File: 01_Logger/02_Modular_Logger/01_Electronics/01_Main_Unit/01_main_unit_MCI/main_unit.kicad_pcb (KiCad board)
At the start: 4 copper layers, 54.9 x 27.4 mm, 34 parts, among them J1 Conn_01x02, J102 FTS-107-01-F-D, J2 Conn_01x04_Pin, J3 Conn_01x04_Pin, J301 Conn_01x02, J302 Conn_02x04_Counter_Clockwise, J304 Conn_02x02_Odd_Even, J701 Micro_SD_Card_Det, SW301 SW_Push, U301 MAX16125WTEG00+T, U302 ESP32-S3-WROOM-1U, U303 DS3231MZ, Y301 Crystal

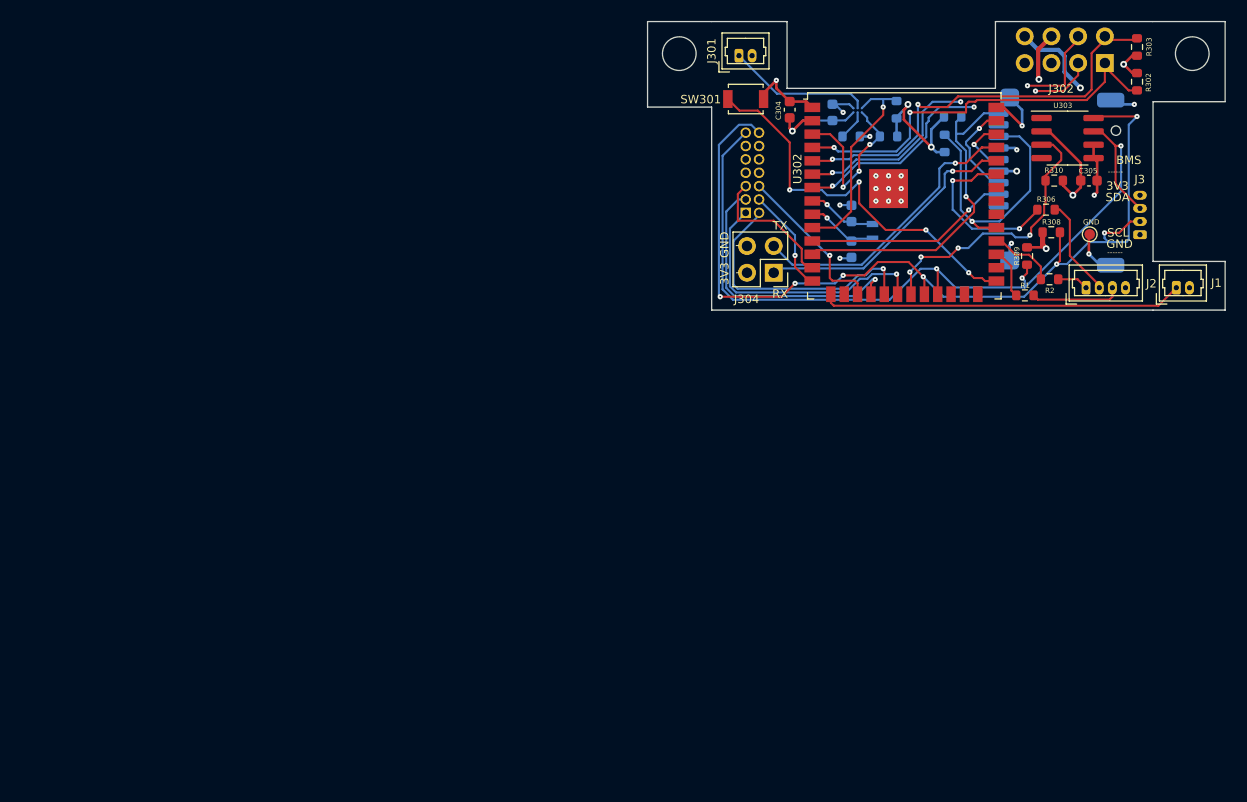
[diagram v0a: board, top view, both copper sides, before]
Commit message: Main_Unit Update
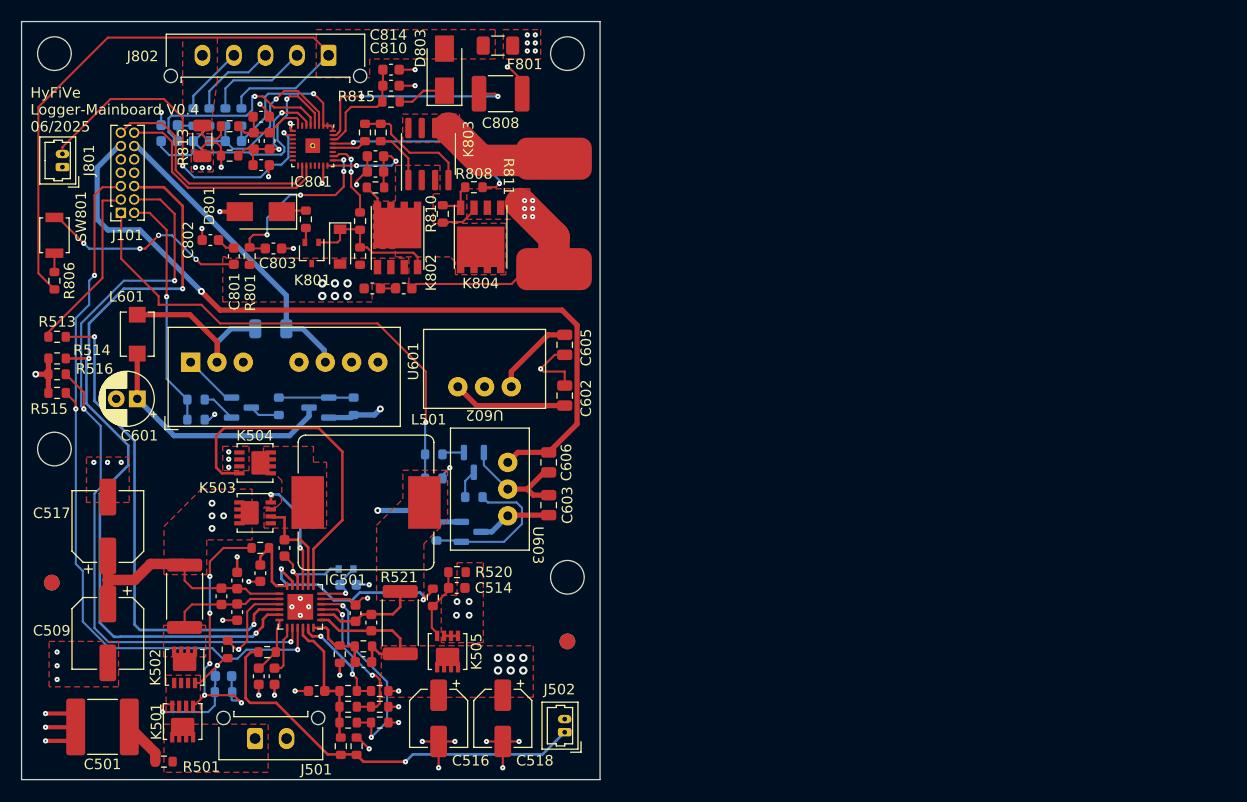
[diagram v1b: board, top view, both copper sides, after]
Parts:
- removed C301, C302: 20pF, Capacitor_SMD:C_0603_1608Metric
- removed C303, C304, C305: 100nF 50V, Capacitor_SMD:C_0603_1608Metric
- removed H303, H305: MountingHole, MountingHole:MountingHole_3.2mm_M3_ISO7380
- removed J1, J301: Conn_01x02, Connector_Molex:Molex_PicoBlade_53047-0210_1x02_P1.25mm_Vertical
- removed J102: FTS-107-01-F-D, Connector_PinHeader_1.27mm:PinHeader_2x07_P1.27mm_Vertical
- removed J2, J3: Conn_01x04_Pin, Connector_Molex:Molex_PicoBlade_53047-0410_1x04_P1.25mm_Vertical
- removed J302: Conn_02x04_Counter_Clockwise, Connector_PinHeader_2.54mm:PinHeader_2x04_P2.54mm_Horizontal
- removed J304: Conn_02x02_Odd_Even, Connector_PinHeader_2.54mm:PinHeader_2x02_P2.54mm_Vertical
- removed J701: Micro_SD_Card_Det, HER_Footprints:SD_CARD_693071020811
- removed R1, R2: 0R, Resistor_SMD:R_0603_1608Metric
- removed R301: 470k, Resistor_SMD:R_0603_1608Metric
- removed R302, R303, R304, R305, R308, R309, R310, R701, R702: 10k, Resistor_SMD:R_0603_1608Metric
- removed R306: 68R, Resistor_SMD:R_0603_1608Metric
- removed SW301: SW_Push, Button_Switch_SMD:SW_SPST_B3U-1000P
- removed TP303: TestPoint, TestPoint:TestPoint_Pad_D1.0mm
- removed U301: MAX16125WTEG00+T, MAX6071ANT25_T:WLP-6
- removed U302: ESP32-S3-WROOM-1U, HER_Footprints:ESP32-S3-WROOM-1U
- removed U303: DS3231MZ, Package_SO:SOIC-8_3.9x4.9mm_P1.27mm
- removed Y301: Crystal, Crystal:Crystal_SMD_TXC_9HT11-2Pin_2.0x1.2mm
- added C501: 47µF 35V X7R, Capacitor_SMD:C_2220_5650Metric, F.Cu at (107.7, 145.3)
- added C502: 100nF 50V, Capacitor_SMD:C_0603_1608Metric, B.Cu at (119.2, 140.5)
- added C503: 100nF 50V, Capacitor_SMD:C_0603_1608Metric, F.Cu at (120.5, 134.4)
- added C504: 1µF 10V, Capacitor_SMD:C_0603_1608Metric, F.Cu at (128.1, 141.9)
- added C505: 100nF 50V, Capacitor_SMD:C_0603_1608Metric, F.Cu at (119.0, 132.9)
- added C506: 100nF 50V, Capacitor_SMD:C_0603_1608Metric, F.Cu at (122.5, 140.5)
- added C507: 100nF 50V, Capacitor_SMD:C_0603_1608Metric, F.Cu at (120.5, 131.4)
- added C508: 33nF 25V, Capacitor_SMD:C_0603_1608Metric, F.Cu at (124.0, 140.5)
- added C509: 47µF 35V, Capacitor_SMD:CP_Elec_6.3x5.4, F.Cu at (108.2, 136.4)
- added C510: 1µF 35V, Capacitor_SMD:C_0603_1608Metric, F.Cu at (122.7, 130.7)
- added C511: 100nF 50V, Capacitor_SMD:C_0603_1608Metric, F.Cu at (125.0, 128.3)
- added C512: 1µF 35V, Capacitor_SMD:C_0603_1608Metric, B.Cu at (131.1, 131.8)
- added C513: 100nF 50V, Capacitor_SMD:C_0603_1608Metric, F.Cu at (131.8, 134.5)
- added C514: 100nF 50V, Capacitor_SMD:C_0603_1608Metric, F.Cu at (141.4, 132.1)
- added C515: 100nF 50V, Capacitor_SMD:C_0603_1608Metric, F.Cu at (133.2, 135.4)
- added C516: 20µF 35V, Capacitor_SMD:CP_Elec_5x5.3, F.Cu at (139.7, 144.5)
- added C517: 47µF 35V, Capacitor_SMD:CP_Elec_6.3x5.4, F.Cu at (108.2, 126.2)
- added C518: 20µF 35V, Capacitor_SMD:CP_Elec_5x5.3, F.Cu at (145.8, 144.5)
- added C519: 22pF 35V, Capacitor_SMD:C_0603_1608Metric, F.Cu at (132.5, 139.1)
- added C601: 10µF, 50V, Capacitor_THT:CP_Radial_D5.0mm_P2.00mm, F.Cu at (111.0, 114.1)
- added C602: 22µF 30V, Capacitor_SMD:C_0805_2012Metric, F.Cu at (151.6, 113.8)
- added C603: 22µF 30V, Capacitor_SMD:C_0805_2012Metric, F.Cu at (150.1, 124.2)
- added C604: 150pF, 2kV, Capacitor_SMD:C_1206_3216Metric, B.Cu at (123.7, 107.4)
- added C605: 47µF 10V, Capacitor_SMD:C_0805_2012Metric, F.Cu at (151.6, 109.0)
- added C606: 47µF 10V, Capacitor_SMD:C_0805_2012Metric, F.Cu at (150.1, 120.1)
- added C801: 100nF 50V, Capacitor_SMD:C_0603_1608Metric, F.Cu at (120.2, 100.5)
- added C802: 100nF 50V, Capacitor_SMD:C_0603_1608Metric, F.Cu at (117.9, 99.0)
- added C803: 10nF, 50V, Capacitor_SMD:C_0603_1608Metric, F.Cu at (123.9, 99.8)
- added C804: 100pF 50V, Capacitor_SMD:C_0603_1608Metric, F.Cu at (133.6, 92.5)
- added C805: 100pF 50V, Capacitor_SMD:C_0603_1608Metric, F.Cu at (133.6, 91.0)
- added C806: 100nF 50V, Capacitor_SMD:C_0603_1608Metric, F.Cu at (133.3, 103.6)
- added C807: 100nF 50V, Capacitor_SMD:C_0603_1608Metric, F.Cu at (136.3, 103.6)
- added C808: 2,2µF 100V, Capacitor_SMD:C_1812_4532Metric, F.Cu at (145.5, 85.1)
- added C809: 100nF 50V, Capacitor_SMD:C_0603_1608Metric, F.Cu at (122.8, 91.9)
- added C810: 100pF 50V, Capacitor_SMD:C_0603_1608Metric, F.Cu at (135.1, 84.3)
- added C811: 100pF 100V, Capacitor_SMD:C_0603_1608Metric, F.Cu at (123.6, 89.6)
- added C812: 100nF 50V, Capacitor_SMD:C_0603_1608Metric, F.Cu at (122.1, 89.6)
- added C813: 100nF 50V, Capacitor_SMD:C_0603_1608Metric, F.Cu at (122.8, 87.3)
- added C814: 100pF 50V, Capacitor_SMD:C_0603_1608Metric, F.Cu at (135.1, 82.8)
- added C815: 100nF 50V, Capacitor_SMD:C_0603_1608Metric, B.Cu at (120.1, 89.6)
- added C816: 100nF 50V, Capacitor_SMD:C_0603_1608Metric, B.Cu at (117.1, 89.6)
- added C817: 100nF 50V, Capacitor_SMD:C_0603_1608Metric, B.Cu at (114.0, 89.6)
- added C818: 100nF 50V, Capacitor_SMD:C_0603_1608Metric, B.Cu at (114.0, 88.1)
- added D501: BAT54W, Diode_SMD:D_SOD-523, B.Cu at (130.8, 130.3)
- added D801: SS1H10-E3/61T, Diode_SMD:D_SMA, F.Cu at (122.7, 96.3)
- added D802: MMSZ5246B-7-F, Diode_SMD:D_SOD-123, F.Cu at (130.3, 99.6)
- added D803: SS1H10-E3/61T, Diode_SMD:D_SMA, F.Cu at (140.2, 82.8)
- added F801: 12A, Fuse:Fuse_1206_3216Metric, F.Cu at (145.3, 80.5)
- added FID301: Fiducial, Sonstiges:Passmarke, F.Cu at (151.9, 137.2)
- added FID302: Fiducial, Sonstiges:Passmarke, F.Cu at (102.9, 131.6)
- added FID303: Fiducial, Sonstiges:Passmarke, B.Cu at (102.9, 131.6)
- added FID304: Fiducial, Sonstiges:Passmarke, B.Cu at (151.9, 137.2)
- added H301: MountingHole, MountingHole:MountingHole_3.2mm_M3_ISO7380, F.Cu at (103.1, 81.3)
- added H302: MountingHole, MountingHole:MountingHole_3.2mm_M3_ISO7380, F.Cu at (151.9, 81.3)
- added H304: MountingHole, MountingHole:MountingHole_3.2mm_M3_ISO7380, F.Cu at (151.9, 131.1)
- added H306: MountingHole, MountingHole:MountingHole_3.2mm_M3_ISO7380, F.Cu at (103.1, 118.9)
- added IC501: BQ24618, Package_DFN_QFN:VQFN-24-1EP_4x4mm_P0.5mm_EP2.45x2.45mm, F.Cu at (126.5, 133.9)
- added IC801: BQ40Z80, Texas:RSM32 VQFN-32-1EP_4x4mm_P0.4mm_EP1.4x1.4mm_ThermalVias, F.Cu at (127.7, 90.0)
- added J101: SFMC-107-01-L-D, Connector_PinSocket_1.27mm:PinSocket_2x07_P1.27mm_Vertical, F.Cu at (109.4, 96.4)
- added J501: Conn_01x02, Connector_Molex:Molex_Micro-Fit_3.0_43650-0215_1x02_P3.00mm_Vertical, F.Cu at (122.2, 146.4)
- added J502: Conn_01x02_Female, Connector_Molex:Molex_PicoBlade_53047-0210_1x02_P1.25mm_Vertical, F.Cu at (151.6, 145.8)
- added J801: Conn_01x02_Male, Connector_Molex:Molex_PicoBlade_53047-0210_1x02_P1.25mm_Vertical, F.Cu at (103.9, 92.1)
- added J802: Conn_01x05_Male, Connector_Molex:Molex_Micro-Fit_3.0_43650-0515_1x05_P3.00mm_Vertical, F.Cu at (129.2, 81.4)
- added K501: SISH101DN-T1-GE3, Vishay:PowerPAK 1212-8 Single, F.Cu at (115.3, 144.8)
- added K502: SISH101DN-T1-GE3, Vishay:PowerPAK 1212-8 Single, F.Cu at (115.5, 139.6)
- added K503: SiS412DN, Vishay:PowerPAK 1212-8 Single, F.Cu at (122.2, 124.9)
- added K504: SiS412DN, Vishay:PowerPAK 1212-8 Single, F.Cu at (122.2, 120.2)
- added K505: SISH101DN-T1-GE3, Vishay:PowerPAK 1212-8 Single, F.Cu at (140.5, 138.1)
- added K801: 2N7002KW, Package_TO_SOT_SMD:SOT-323_SC-70, F.Cu at (127.6, 100.2)
- added K802: CSD18540Q5B, HER_Footprints:TI Q5B-Package, F.Cu at (135.7, 98.8)
- added K803: DMP6023LSS-13, Package_SO:SOIC-8_3.9x4.9mm_P1.27mm, F.Cu at (138.7, 90.8)
- added K804: CSD18540Q5B, HER_Footprints:TI Q5B-Package, F.Cu at (143.6, 98.7)
- added L501: 3,3µH, Inductor_SMD:L_Bourns_SRP1245A, F.Cu at (132.7, 124.0)
- added L601: 10µH, HER_Footprints:CC453232A, F.Cu at (111.0, 108.0)
- added Q601: BSS123, Package_TO_SOT_SMD:SOT-23, B.Cu at (120.9, 114.9)
- added Q602: IRLML5203TRPBF, Package_TO_SOT_SMD:SOT-23, B.Cu at (128.3, 114.9)
- added Q603: BSS123, Package_TO_SOT_SMD:SOT-23, B.Cu at (143.0, 120.1)
- added Q604: IRLML5203TRPBF, Package_TO_SOT_SMD:SOT-23, B.Cu at (142.7, 126.7)
- added R501: 100R, Resistor_SMD:R_0603_1608Metric, F.Cu at (113.5, 148.6)
- added R502: 10k, Resistor_SMD:R_0603_1608Metric, F.Cu at (131.0, 144.9)
- added R503: 5.7k, Resistor_SMD:R_0603_1608Metric, F.Cu at (134.0, 144.9)
- added R504: R_Therm_1, Resistor_SMD:R_0603_1608Metric, F.Cu at (130.3, 147.1)
- added R505: R_Therm_2, Resistor_SMD:R_0603_1608Metric, F.Cu at (131.8, 147.1)
- added R506: 100k, Resistor_SMD:R_0603_1608Metric, F.Cu at (131.1, 143.4)
- added R507: 10k, Resistor_SMD:R_0603_1608Metric, F.Cu at (134.0, 143.4)
- added R508: 232k, Resistor_SMD:R_0603_1608Metric, F.Cu at (131.1, 141.9)
- added R509: 33k, Resistor_SMD:R_0603_1608Metric, F.Cu at (134.1, 141.9)
- added R510: 100k, Resistor_SMD:R_0603_1608Metric, B.Cu at (119.2, 142.0)
- added R511: 100R, Resistor_SMD:R_0603_1608Metric, F.Cu at (123.3, 138.2)
- added R512: 1k, Resistor_SMD:R_0603_1608Metric, F.Cu at (119.6, 137.9)
- added R513: 0R, Resistor_SMD:R_0603_1608Metric, F.Cu at (103.4, 108.2)
- added R514: 49,9k, Resistor_SMD:R_0603_1608Metric, F.Cu at (103.4, 110.3)
- added R515: 49,9k, Resistor_SMD:R_0603_1608Metric, F.Cu at (103.4, 113.5)
- added R516: 49,9k, Resistor_SMD:R_0603_1608Metric, F.Cu at (103.4, 111.8)
- added R517: 10m, Resistor_SMD:R_2512_6332Metric, F.Cu at (115.5, 132.9)
- added R518: 10R, Resistor_SMD:R_0603_1608Metric, F.Cu at (122.7, 128.3)
- added R519: 1k, Resistor_SMD:R_0603_1608Metric, F.Cu at (139.1, 133.0)
- added R520: 100k, Resistor_SMD:R_0603_1608Metric, F.Cu at (141.4, 130.6)
- added R521: 10m, Resistor_SMD:R_2512_6332Metric, F.Cu at (136.0, 135.4)
- added R522: 357k, Resistor_SMD:R_0603_1608Metric, F.Cu at (132.5, 137.6)
- added R523: 49,9k, Resistor_SMD:R_0603_1608Metric, F.Cu at (130.2, 138.4)
- added R601: 2k7, Resistor_SMD:R_0603_1608Metric, B.Cu at (116.6, 116.1)
- added R602: 47k, Resistor_SMD:R_0603_1608Metric, B.Cu at (116.6, 114.2)
- added R603: 680k, Resistor_SMD:R_0603_1608Metric, B.Cu at (131.6, 114.8)
- added R604: 1k, Resistor_SMD:R_0603_1608Metric, B.Cu at (124.5, 114.8)
- added R605: 2k7, Resistor_SMD:R_0603_1608Metric, B.Cu at (139.2, 121.7)
- added R606: 47k, Resistor_SMD:R_0603_1608Metric, B.Cu at (139.2, 119.4)
- added R607: 680k, Resistor_SMD:R_0603_1608Metric, B.Cu at (139.4, 126.7)
- added R608: 1k, Resistor_SMD:R_0603_1608Metric, B.Cu at (143.0, 123.4)
- added R801: 1,1k, Resistor_SMD:R_0603_1608Metric, F.Cu at (121.7, 100.5)
- added R802: 10k, Resistor_SMD:R_0603_1608Metric, F.Cu at (127.0, 97.0)
- added R803: 10M, Resistor_SMD:R_0603_1608Metric, F.Cu at (132.2, 100.5)
- added R804: 4,81k, Resistor_SMD:R_0603_1608Metric, F.Cu at (132.2, 97.2)
- added R805: 510R, Resistor_SMD:R_0603_1608Metric, F.Cu at (133.6, 94.0)
- added R806: 51R, Resistor_SMD:R_0603_1608Metric, F.Cu at (103.1, 102.9)
- added R807: 10M, Resistor_SMD:R_0603_1608Metric, F.Cu at (134.1, 88.8)
- added R808: 1k, Resistor_SMD:R_0603_1608Metric, F.Cu at (143.0, 94.0)
- added R809: 10k, Resistor_SMD:R_0603_1608Metric, F.Cu at (132.6, 88.8)
- added R810: 10M, Resistor_SMD:R_0603_1608Metric, F.Cu at (140.0, 96.5)
- added R811: 46.4 5W, Sonstiges:R_4527_11570Metric, F.Cu at (150.6, 96.5)
- added R812: 100R, Resistor_SMD:R_0603_1608Metric, F.Cu at (119.8, 91.0)
- added R813: 1m, Resistor_SMD:R_1206_3216Metric, F.Cu at (117.2, 89.6)
- added R814: 100R, Resistor_SMD:R_0603_1608Metric, F.Cu at (119.8, 88.2)
- added R815: 100R, Resistor_SMD:R_0603_1608Metric, F.Cu at (135.1, 85.9)
- added R816: 499R, Resistor_SMD:R_0603_1608Metric, B.Cu at (120.9, 87.3)
- added R817: 499R, Resistor_SMD:R_0603_1608Metric, B.Cu at (119.4, 87.3)
- added R818: 499R, Resistor_SMD:R_0603_1608Metric, B.Cu at (117.9, 87.3)
- added R819: 499R, Resistor_SMD:R_0603_1608Metric, B.Cu at (116.3, 87.3)
- added SW801: SW_Push, Button_Switch_SMD:SW_SPST_B3U-1000P, F.Cu at (103.1, 98.6)
- added U601: SPBW06F-12, Converter_DCDC:Converter_DCDC_XP_POWER-ITxxxxxS_THT, F.Cu at (116.1, 110.6)
- added U602: OKI-78SR-3.3_1.5-W36-C, HER_Footprints:DC_DC_Converter, F.Cu at (144.0, 113.0)
- added U603: OKI-78SR-5_1.5-W36-C, HER_Footprints:DC_DC_Converter, F.Cu at (146.2, 122.7)
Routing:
- net /power/System+: track 0.00 -> 128.4 mm, vias 0 -> 10
- net /power/BMS/PACK+: track 0.00 -> 94.1 mm, vias 0 -> 16
- net /MPU/I2C_SMBus_SCL: track 89.6 -> 0.00 mm, vias 7 -> 0
- net /MPU/I2C_SMBus_SDA: track 78.8 -> 0.00 mm, vias 3 -> 0
- net /power/~{PG}: track 0.00 -> 75.9 mm, vias 0 -> 3
- net /power/~{STAT1}: track 0.00 -> 75.9 mm, vias 0 -> 3
- net /power/~{STAT2}: track 0.00 -> 70.8 mm, vias 0 -> 3
- net /power/BMS/BAT_PLUS: track 0.00 -> 59.9 mm
- net /power/ENABLE_5V: track 0.00 -> 48.4 mm, vias 0 -> 1
- net GND: track 36.7 -> 84.2 mm, vias 20 -> 54
- net Net-(IC501-CE): track 0.00 -> 47.0 mm, vias 0 -> 2
- net +3V3: track 58.2 -> 12.5 mm, vias 8 -> 1
- net /MPU/I2C_BUS_CLK: track 39.4 -> 0.00 mm, vias 2 -> 0
- net /power/Battery_Charger/Thermistor: track 0.00 -> 39.3 mm, vias 0 -> 1
- net /power/BMS/BAT_PLUS_F: track 0.00 -> 38.0 mm, vias 0 -> 12
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- added copper zone on F.Cu, net /power/BMS/BAT_MINUS
- added copper zone on F.Cu, net /power/BMS/BAT_PLUS
- added copper zone on F.Cu, net /power/BMS/BAT_PLUS_F
- added copper zone on F.Cu, net /power/BMS/PACK+
- added copper zone on In2.Cu, net /power/BMS/PACK+
- added copper zone on F.Cu, net /power/Battery_Charger/ACP
- added copper zone on F.Cu, net /power/Battery_Charger/VIN
- added copper zone on F.Cu, net /power/System+
- added copper zone on In2.Cu, net /power/System+
- added copper zone on F.Cu, net GND
- added copper zone on F.Cu, net Net-(C502-Pad1)
- added copper zone on F.Cu, net Net-(IC501-PH)
- added copper zone on F.Cu, net Net-(IC501-SRP)
- added copper zone on F.Cu, net Net-(K802-Pad5)
- added copper zone on F.Cu, net Net-(K803-Pad5)
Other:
- board size 54.9 x 27.4 mm -> 55 x 72.1 mm
- board text added: "HyFiVe Logger-Mainboard V0.4 06/2025"
- board text removed: "-"
- board text removed: "------"
- board text removed: "3V3"
- board text removed: "BMS"
- board text removed: "GND"
- board text removed: "HyFiVe Logger-MPU-Board V0.5 08/2025"
- board text removed: "RX"
- board text removed: "SCL"
- board text removed: "SDA"
- board text removed: "TX"
